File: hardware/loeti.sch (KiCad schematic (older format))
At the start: 64 parts, among them J1 GCT USB4105, J2 AudioJack3, J3 20021112-00014T1LF, Q1 BC817, Q2 BC817, Q3 BC807, Q4 Si4825DDY, DMG4435SSS, IRF939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, SW1 D6R, U1 STUSB4500QTR, U2 AP2204R-3.3, U3 STM32F030K6Tx, U4 74AHC1G08, U5 INA301, U6 TMP100, U7 TLV333-DBV

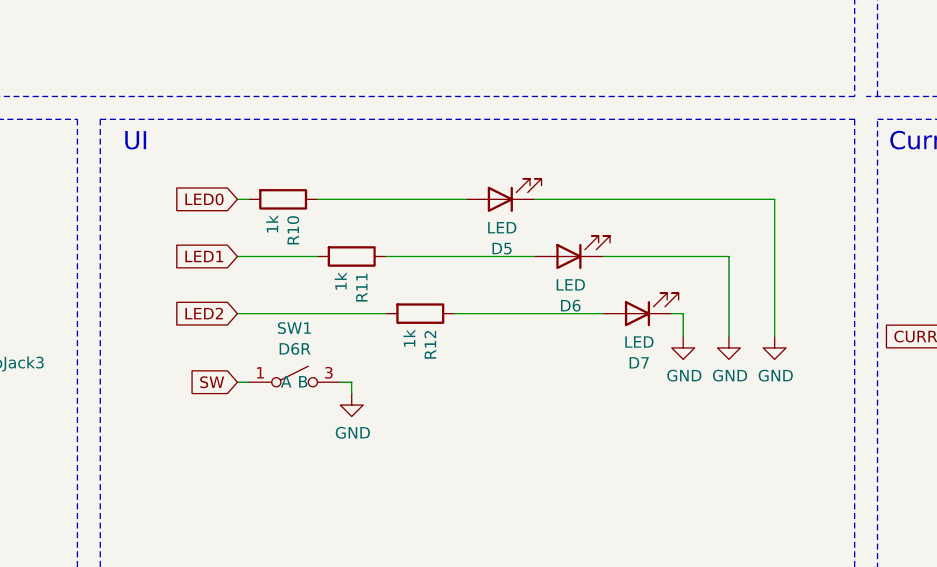
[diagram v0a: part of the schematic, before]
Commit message: two-temperature mode
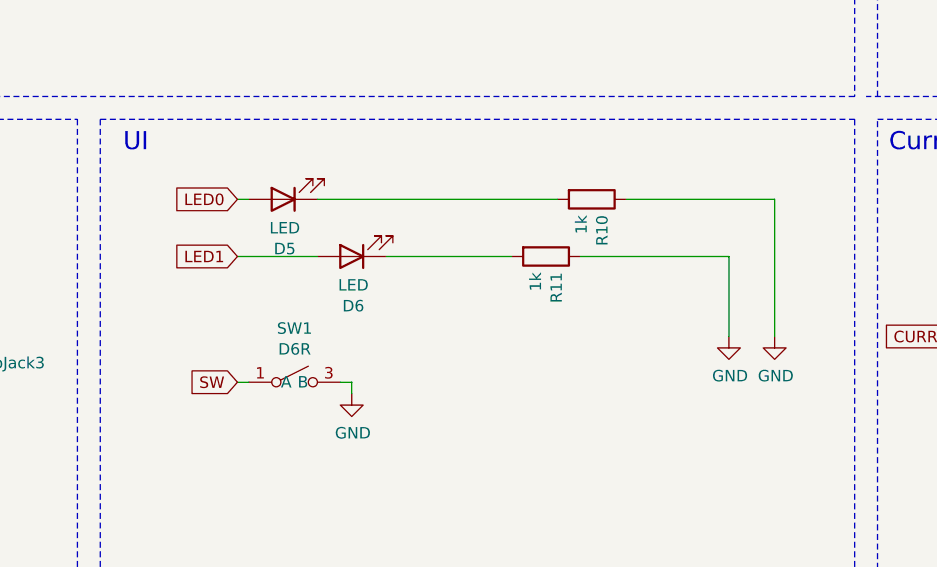
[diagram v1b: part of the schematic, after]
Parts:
- removed D7: LED, LED_THT:LED_D1.8mm_W3.3mm_H2.4mm, symbol Device:LED
- removed R12: 1k, Resistor_SMD:R_0603_1608Metric_Pad0.98x0.95mm_HandSolder, symbol Device:R
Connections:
- net GND: now also R10.1, R11.1; no longer D5.1 (K), D6.1 (K)
- net LED0: now also D5.2 (A); no longer R10.2
- net LED1: now also D6.2 (A); no longer R11.2
- new net: D5.1 (K), R10.2
- new net: D6.1 (K), R11.2
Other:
- moved on the sheet: D5, D6, R10, R11
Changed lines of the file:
@@
 LED0
-$Comp
-L Device:LED D5
-U 1 1 60A6F838
-P 8600 8200
-F 0 "D5" H 8593 8417 50  0000 C CNN
-F 1 "LED" H 8593 8326 50  0000 C CNN
-F 2 "LED_THT:LED_D1.8mm_W3.3mm_H2.4mm" H 8600 8200 50  0001 C CNN
-F 3 "~" H 8600 8200 50  0001 C CNN
-	1    8600 8200
-	-1   0    0    1
-$EndComp
-Wire Wire Line
-	8750 8200 9800 8200
-Wire Wire Line
-	9050 8450 9600 8450
-Wire Wire Line
-	9400 8700 9350 8700
-Wire Wire Line
-	9400 8800 9400 8700
 $Comp
 L power:GND #PWR036
@@
 	1    0    0    -1
 $EndComp
-$Comp
-L power:GND #PWR034
-U 1 1 60AE7307
-P 9400 8800
-F 0 "#PWR034" H 9400 8550 50  0001 C CNN
-F 1 "GND" H 9405 8627 50  0000 C CNN
-F 2 "" H 9400 8800 50  0001 C CNN
-F 3 "" H 9400 8800 50  0001 C CNN
-	1    9400 8800
-	1    0    0    -1
-$EndComp
-Wire Wire Line
-	8400 8700 9050 8700
-$Comp
-L Device:LED D7
-U 1 1 60A95747
-P 9200 8700
-F 0 "D7" H 9193 8917 50  0000 C CNN
-F 1 "LED" H 9193 8826 50  0000 C CNN
-F 2 "LED_THT:LED_D1.8mm_W3.3mm_H2.4mm" H 9200 8700 50  0001 C CNN
-F 3 "~" H 9200 8700 50  0001 C CNN
-	1    9200 8700
-	-1   0    0    1
-$EndComp
-$Comp
-L Device:LED D6
-U 1 1 60A952E3
-P 8900 8450
-F 0 "D6" H 8893 8667 50  0000 C CNN
-F 1 "LED" H 8893 8576 50  0000 C CNN
-F 2 "LED_THT:LED_D1.8mm_W3.3mm_H2.4mm" H 8900 8450 50  0001 C CNN
-F 3 "~" H 8900 8450 50  0001 C CNN
-	1    8900 8450
-	-1   0    0    1
-$EndComp
 Wire Wire Line
 	7500 9000 7450 9000
@@
 	1    0    0    -1
 $EndComp
-Wire Wire Line
-	8100 8450 8750 8450
-$Comp
-L Device:R R12
-U 1 1 60AC0274
-P 8250 8700
-F 0 "R12" H 8319 8746 50  0000 L CNN
-F 1 "1k" H 8319 8655 50  0000 L CNN
-F 2 "Resistor_SMD:R_0603_1608Metric_Pad0.98x0.95mm_HandSolder" V 8180 8700 50  0001 C CNN
-F 3 "~" H 8250 8700 50  0001 C CNN
-	1    8250 8700
-	0    1    1    0
-$EndComp
-$Comp
-L Device:R R11
-U 1 1 60ABFEAA
-P 7950 8450
-F 0 "R11" H 8019 8496 50  0000 L CNN
-F 1 "1k" H 8019 8405 50  0000 L CNN
-F 2 "Resistor_SMD:R_0603_1608Metric_Pad0.98x0.95mm_HandSolder" V 7880 8450 50  0001 C CNN
-F 3 "~" H 7950 8450 50  0001 C CNN
-	1    7950 8450
-	0    1    1    0
-$EndComp
-Wire Wire Line
-	7450 8700 8100 8700
-Wire Wire Line
-	7450 8450 7800 8450
-Text GLabel 7450 8700 0    50   Input ~ 0
-LED2
 Text GLabel 7450 8450 0    50   Input ~ 0
 LED1
-Wire Wire Line
-	8450 8200 7800 8200
-$Comp
-L Device:R R10
-U 1 1 60ABF026
-P 7650 8200
-F 0 "R10" H 7719 8246 50  0000 L CNN
-F 1 "1k" H 7719 8155 50  0000 L CNN
-F 2 "Resistor_SMD:R_0603_1608Metric_Pad0.98x0.95mm_HandSolder" V 7580 8200 50  0001 C CNN
-F 3 "~" H 7650 8200 50  0001 C CNN
-	1    7650 8200
-	0    1    1    0
-$EndComp
 Wire Wire Line
 	7450 8200 7500 8200
@@
 Text Notes 5250 8550 0    50   ~ 0
 Only C245\nSleeve: green (TC-, heater)\nRing: red (TC+)\nTip: blue (heater)
+$Comp
+L Device:LED D5
+U 1 1 60A6F838
+P 7650 8200
+F 0 "D5" H 7643 8417 50  0000 C CNN
+F 1 "LED" H 7643 8326 50  0000 C CNN
+F 2 "LED_THT:LED_D1.8mm_W3.3mm_H2.4mm" H 7650 8200 50  0001 C CNN
+F 3 "~" H 7650 8200 50  0001 C CNN
+	1    7650 8200
+	-1   0    0    1
+$EndComp
+Wire Wire Line
+	7800 8200 8850 8200
+Wire Wire Line
+	8100 8450 8650 8450
+$Comp
+L Device:LED D6
+U 1 1 60A952E3
+P 7950 8450
+F 0 "D6" H 7943 8667 50  0000 C CNN
+F 1 "LED" H 7943 8576 50  0000 C CNN
+F 2 "LED_THT:LED_D1.8mm_W3.3mm_H2.4mm" H 7950 8450 50  0001 C CNN
+F 3 "~" H 7950 8450 50  0001 C CNN
+	1    7950 8450
+	-1   0    0    1
+$EndComp
+Wire Wire Line
+	7800 8450 7450 8450
+Wire Wire Line
+	9800 8200 9150 8200
+$Comp
+L Device:R R10
+U 1 1 60ABF026
+P 9000 8200
+F 0 "R10" H 9069 8246 50  0000 L CNN
+F 1 "1k" H 9069 8155 50  0000 L CNN
+F 2 "Resistor_SMD:R_0603_1608Metric_Pad0.98x0.95mm_HandSolder" V 8930 8200 50  0001 C CNN
+F 3 "~" H 9000 8200 50  0001 C CNN
+	1    9000 8200
+	0    1    1    0
+$EndComp
+$Comp
+L Device:R R11
+U 1 1 60ABFEAA
+P 8800 8450
+F 0 "R11" H 8869 8496 50  0000 L CNN
+F 1 "1k" H 8869 8405 50  0000 L CNN
+F 2 "Resistor_SMD:R_0603_1608Metric_Pad0.98x0.95mm_HandSolder" V 8730 8450 50  0001 C CNN
+F 3 "~" H 8800 8450 50  0001 C CNN
+	1    8800 8450
+	0    1    1    0
+$EndComp
+Wire Wire Line
+	8950 8450 9600 8450
 $EndSCHEMATC
